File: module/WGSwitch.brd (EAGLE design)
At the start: 32.7 x 55.5 mm, 34 parts, among them Q1 MMBT3904, Q2 MMBT3904, Q3 MMBT3904, Q4 PMBT3906, U1 7805TV, U2 ARDUINO_PRO_MINI

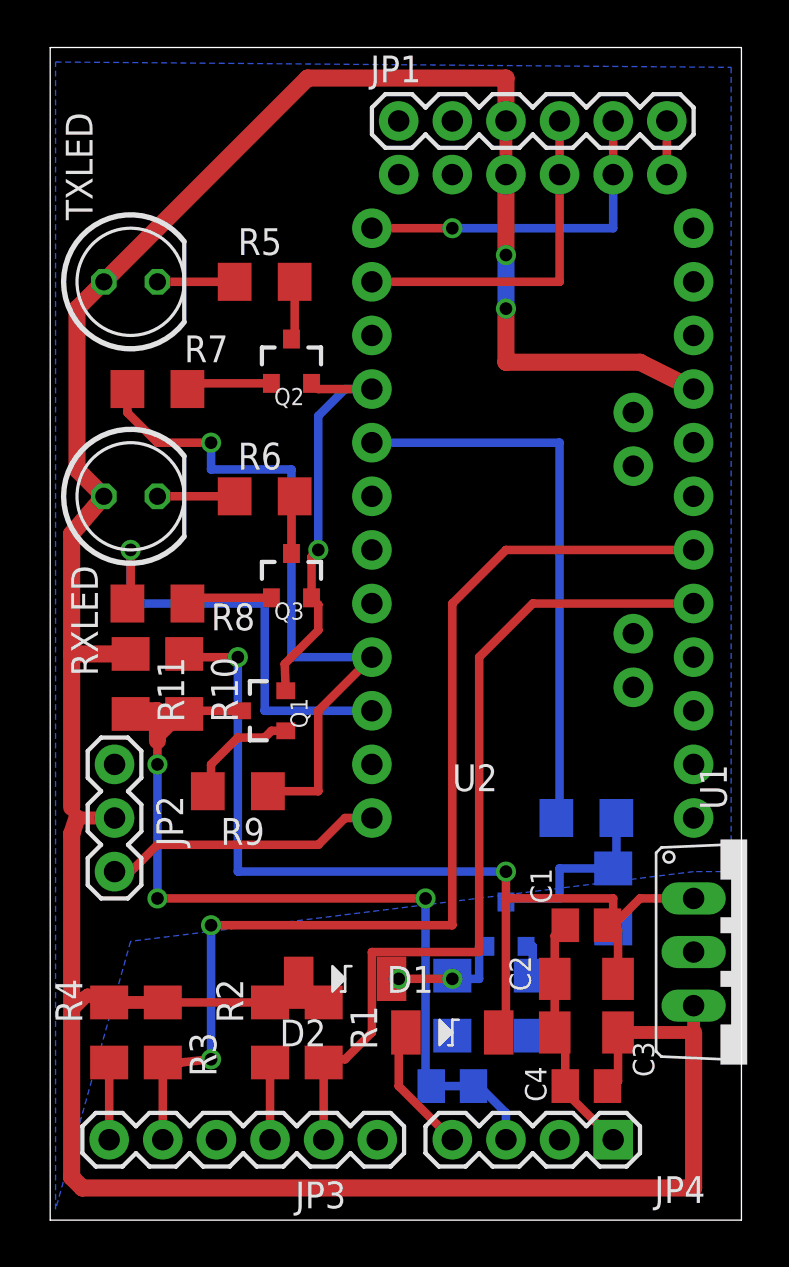
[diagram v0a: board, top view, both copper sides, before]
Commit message: Just about right.
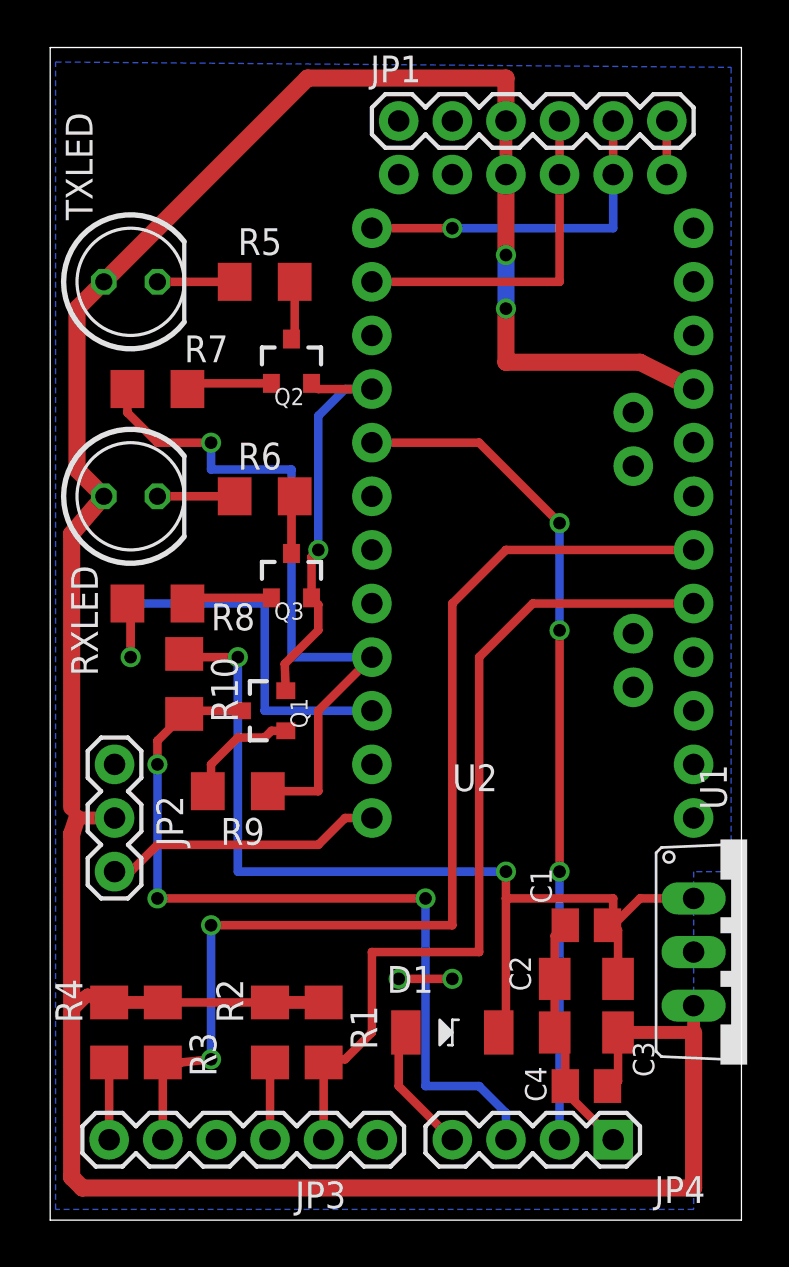
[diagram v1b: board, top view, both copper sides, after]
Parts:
- removed C5: 0.1, rcl:C0805K
- removed D2: PMEG3030EP, kb1vc_robot_parts:SOD128
- removed Q4: PMBT3906, SparkFun-DiscreteSemi:SOT23-3
- removed R11, R12, R13, R14, R15: 10K, rcl:R1206
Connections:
- removed net N$12: Q4.3, R14.2, R15.2
- removed net N$5: D2.P$2, Q4.2, R12.2
- removed net N$9: Q4.1, R13.1
- removed net PTT_H: R15.1, U2.5
- removed net PTT_IN_RAW_L: C5.1, JP4.2, R12.1, R13.2
- new net PTT_IN_L: JP4.2, U2.5
- net GND: no longer C5.2, R14.1
- net TX_EN_OUT_L: no longer R11.2
- net VCC: no longer D2.P$1, R11.1
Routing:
- net PTT_IN_L: track 0.00 -> 39.7 mm, vias 0 -> 3
- net PTT_H: track 26.8 -> 0.00 mm
- net N$12: track 9.21 -> 0.00 mm
- net N$5: track 3.28 -> 0.00 mm
- net TX_EN_OUT_L: track 42.1 -> 39.2 mm
- net VCC: track 152.3 -> 149.5 mm
- net N$9: track 1.71 -> 0.00 mm
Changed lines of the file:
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@@
 <?xml version="1.0" encoding="utf-8"?>
 <!DOCTYPE eagle SYSTEM "eagle.dtd">
-<eagle version="7.3.0">
+<eagle version="7.5.0">
 <drawing>
 <settings>
@@
 <layer number="19" name="Unrouted" color="6" fill="1" visible="yes" active="yes"/>
 <layer number="20" name="Dimension" color="15" fill="1" visible="yes" active="yes"/>
-<layer number="21" name="tPlace" color="7" fill="1" visible="no" active="yes"/>
-<layer number="22" name="bPlace" color="7" fill="1" visible="no" active="yes"/>
+<layer number="21" name="tPlace" color="7" fill="1" visible="yes" active="yes"/>
+<layer number="22" name="bPlace" color="7" fill="1" visible="yes" active="yes"/>
 <layer number="23" name="tOrigins" color="15" fill="1" visible="yes" active="yes"/>
 <layer number="24" name="bOrigins" color="15" fill="1" visible="yes" active="yes"/>
@@
 <attribute name="VALUE" x="25.4" y="17.78" size="1.27" layer="27" ratio="10" rot="R270"/>
 </element>
-<element name="R11" library="rcl" package="R1206" value="10K" x="3.81" y="25.4" rot="R270"/>
-<element name="Q4" library="SparkFun-DiscreteSemi" package="SOT23-3" value="PMBT3906" x="21.59" y="13.97" rot="MR0">
-<attribute name="PROD_ID" value="TRANS-08052" x="21.59" y="13.97" size="1.778" layer="28" rot="MR0" display="off"/>
-</element>
-<element name="D2" library="kb1vc_robot_parts" package="SOD128" value="PMEG3030EP" x="13.97" y="11.43"/>
-<element name="R12" library="rcl" package="R1206" value="10K" x="19.05" y="10.16" rot="MR90"/>
-<element name="R13" library="rcl" package="R1206" value="10K" x="22.86" y="10.16" rot="MR270"/>
-<element name="C5" library="rcl" package="C0805K" value="0.1" x="19.05" y="6.35" rot="MR0"/>
-<element name="R14" library="rcl" package="R1206" value="10K" x="26.67" y="15.24" rot="MR90"/>
-<element name="R15" library="rcl" package="R1206" value="10K" x="25.4" y="19.05" rot="MR180"/>
 </elements>
 <signals>
@@
 <vertex x="32.258" y="16.51"/>
 <vertex x="30.48" y="16.51"/>
-<vertex x="3.81" y="13.208"/>
+<vertex x="30.48" y="0.508"/>
 <vertex x="0.254" y="0.508"/>
 </polygon>
@@
 <via x="19.05" y="11.43" extent="1-16" drill="0.6" shape="square"/>
 <wire x1="16.51" y1="11.43" x2="19.05" y2="11.43" width="0.4064" layer="1"/>
-<contactref element="C5" pad="2"/>
-<contactref element="R14" pad="1"/>
-<wire x1="26.67" y1="13.818" x2="30.48" y2="12.7" width="0" layer="19" extent="16-16"/>
-<wire x1="24.4" y1="13.97" x2="26.67" y2="13.818" width="0" layer="19" extent="1-16"/>
-<wire x1="19.05" y1="11.43" x2="23.9" y2="11.43" width="0" layer="19" extent="1-1"/>
-<wire x1="18.05" y1="6.35" x2="19.05" y2="11.43" width="0" layer="19" extent="16-16"/>
-<wire x1="15.494" y1="3.81" x2="18.05" y2="6.35" width="0" layer="19" extent="16-16"/>
-<wire x1="7.874" y1="3.81" x2="15.494" y2="3.81" width="0" layer="19" extent="1-1"/>
-<wire x1="11.16" y1="25.08" x2="16.51" y2="11.43" width="0" layer="19" extent="1-1"/>
 </signal>
 <signal name="VCC">
@@
 <wire x1="3.048" y1="19.05" x2="1.27" y2="19.05" width="0.6096" layer="1"/>
 <wire x1="1.27" y1="19.05" x2="1.016" y2="19.558" width="0.6096" layer="1"/>
-<wire x1="1.016" y1="19.558" x2="1.016" y2="26.822" width="0.8128" layer="1"/>
-<wire x1="1.016" y1="26.822" x2="1.016" y2="32.512" width="0.8128" layer="1"/>
+<wire x1="1.016" y1="19.558" x2="1.016" y2="32.512" width="0.8128" layer="1"/>
 <wire x1="1.016" y1="32.512" x2="2.54" y2="34.29" width="0.8128" layer="1"/>
 <wire x1="2.54" y1="44.45" x2="12.192" y2="54.102" width="0.8128" layer="1"/>
@@
 <wire x1="1.016" y1="9.906" x2="1.778" y2="10.668" width="0.6096" layer="1"/>
 <wire x1="5.334" y1="10.312" x2="10.414" y2="10.312" width="0.4064" layer="1"/>
-<contactref element="R11" pad="1"/>
-<wire x1="3.81" y1="26.822" x2="1.016" y2="26.822" width="0.8128" layer="1"/>
-<contactref element="D2" pad="P$1"/>
-<wire x1="12.954" y1="10.312" x2="11.77" y2="11.43" width="0" layer="19" extent="1-1"/>
 </signal>
 <signal name="N$10">
@@
 <contactref element="R8" pad="1"/>
 <contactref element="U2" pad="10"/>
-<via x="3.81" y="31.75" extent="1-16" drill="0.6" shape="square"/>
-<wire x1="3.81" y1="31.75" x2="3.81" y2="29.058" width="0.4064" layer="1"/>
+<via x="3.81" y="26.67" extent="1-16" drill="0.6" shape="square"/>
+<wire x1="3.81" y1="26.67" x2="3.81" y2="29.058" width="0.4064" layer="1"/>
 <wire x1="3.81" y1="29.058" x2="3.658" y2="29.21" width="0.4064" layer="1"/>
-<wire x1="3.81" y1="31.75" x2="3.81" y2="29.21" width="0.4064" layer="16"/>
+<wire x1="3.81" y1="26.67" x2="3.81" y2="29.21" width="0.4064" layer="16"/>
 <wire x1="3.81" y1="29.21" x2="10.16" y2="29.21" width="0.4064" layer="16"/>
 <wire x1="10.16" y1="29.21" x2="10.16" y2="24.13" width="0.4064" layer="16"/>
@@
 <wire x1="7.62" y1="36.83" x2="5.08" y2="36.83" width="0.4064" layer="1"/>
 <wire x1="5.08" y1="36.83" x2="3.658" y2="38.252" width="0.4064" layer="1"/>
+</signal>
+<signal name="PTT_IN_L">
+<contactref element="JP4" pad="2"/>
+<contactref element="U2" pad="5"/>
+<wire x1="15.24" y1="36.83" x2="20.32" y2="36.83" width="0.4064" layer="1"/>
+<wire x1="20.32" y1="36.83" x2="24.13" y2="33.02" width="0.4064" layer="1"/>
+<via x="24.13" y="33.02" extent="1-16" drill="0.6" shape="square"/>
+<wire x1="24.13" y1="33.02" x2="24.13" y2="27.94" width="0.4064" layer="16"/>
+<via x="24.13" y="27.94" extent="1-16" drill="0.6" shape="square"/>
+<wire x1="24.13" y1="27.94" x2="24.13" y2="16.51" width="0.4064" layer="1"/>
+<via x="24.13" y="16.51" extent="1-16" drill="0.6" shape="square"/>
+<wire x1="24.13" y1="16.51" x2="24.13" y2="3.81" width="0.4064" layer="16"/>
 </signal>
 <signal name="TX_EN_OUT_L">
@@
 <wire x1="20.32" y1="6.35" x2="21.59" y2="5.08" width="0.4064" layer="16"/>
 <wire x1="21.59" y1="5.08" x2="21.59" y2="3.81" width="0.4064" layer="16"/>
-<contactref element="R11" pad="2"/>
-<wire x1="5.08" y1="22.708" x2="5.08" y2="24.13" width="0.8128" layer="1"/>
-<wire x1="5.08" y1="24.13" x2="3.81" y2="24.13" width="0.8128" layer="1"/>
-<wire x1="3.81" y1="24.13" x2="3.81" y2="23.978" width="0.8128" layer="1"/>
 </signal>
 <signal name="N$2">
@@
 <wire x1="6.772" y1="39.64" x2="6.502" y2="39.37" width="0.4064" layer="1"/>
 </signal>
-<signal name="PTT_IN_RAW_L">
-<contactref element="JP4" pad="2"/>
-<contactref element="R12" pad="1"/>
-<contactref element="C5" pad="1"/>
-<contactref element="R13" pad="2"/>
-<wire x1="20.05" y1="6.35" x2="22.86" y2="8.738" width="0" layer="19" extent="16-16"/>
-<wire x1="19.05" y1="8.738" x2="20.05" y2="6.35" width="0" layer="19" extent="16-16"/>
-<wire x1="24.13" y1="3.81" x2="20.05" y2="6.35" width="0" layer="19" extent="16-16"/>
-</signal>
-<signal name="N$5">
-<contactref element="D2" pad="P$2"/>
-<contactref element="Q4" pad="2"/>
-<contactref element="R12" pad="2"/>
-<wire x1="16.17" y1="11.43" x2="19.05" y2="11.582" width="0" layer="19" extent="1-16"/>
-<wire x1="20.64" y1="12.97" x2="20.32" y2="12.97" width="0.4064" layer="16"/>
-<wire x1="20.32" y1="12.97" x2="20.32" y2="11.43" width="0.4064" layer="16"/>
-<wire x1="20.32" y1="11.43" x2="19.05" y2="11.43" width="0.4064" layer="16"/>
-<wire x1="19.05" y1="11.43" x2="19.05" y2="11.582" width="0.4064" layer="16"/>
-</signal>
-<signal name="N$9">
-<contactref element="Q4" pad="1"/>
-<contactref element="R13" pad="1"/>
-<wire x1="22.54" y1="12.97" x2="22.86" y2="12.97" width="0.4064" layer="16"/>
-<wire x1="22.86" y1="12.97" x2="22.86" y2="11.582" width="0.4064" layer="16"/>
-</signal>
-<signal name="N$12">
-<contactref element="Q4" pad="3"/>
-<contactref element="R14" pad="2"/>
-<contactref element="R15" pad="2"/>
-<wire x1="26.67" y1="16.662" x2="26.822" y2="16.662" width="0.4064" layer="16"/>
-<wire x1="26.822" y1="16.662" x2="26.822" y2="19.05" width="0.4064" layer="16"/>
-<wire x1="26.67" y1="16.662" x2="24.13" y2="16.662" width="0.4064" layer="16"/>
-<wire x1="24.13" y1="16.662" x2="24.13" y2="15.24" width="0.4064" layer="16"/>
-<wire x1="24.13" y1="15.24" x2="21.59" y2="15.24" width="0.4064" layer="16"/>
-<wire x1="21.59" y1="15.24" x2="21.59" y2="15.07" width="0.4064" layer="16"/>
-</signal>
-<signal name="PTT_H">
-<contactref element="R15" pad="1"/>
-<contactref element="U2" pad="5"/>
-<wire x1="23.978" y1="19.05" x2="24.13" y2="19.05" width="0.4064" layer="16"/>
-<wire x1="24.13" y1="19.05" x2="24.13" y2="36.83" width="0.4064" layer="16"/>
-<wire x1="24.13" y1="36.83" x2="15.24" y2="36.83" width="0.4064" layer="16"/>
-</signal>
 </signals>
